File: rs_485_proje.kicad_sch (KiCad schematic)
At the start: 69 parts, among them J1 xt60_female, J10 Extra_pins, J12 P_E_SENSOR_2, J2 RJ45_LED, J3 xt60_female, J4 Led_conn, J5 P_E_SENSOR_1, J6 USB_B_Mini, J7 H_E_sensor_1, J8 H_E_sensor_2, J9 Debug, U1 AP2112K-3.3, U10 FT232RL, U11 USBLC6-2SC6, U2 STM32G030F6Px, U4 ADM2587E, U5 TPS5420D, U7 TLP2161

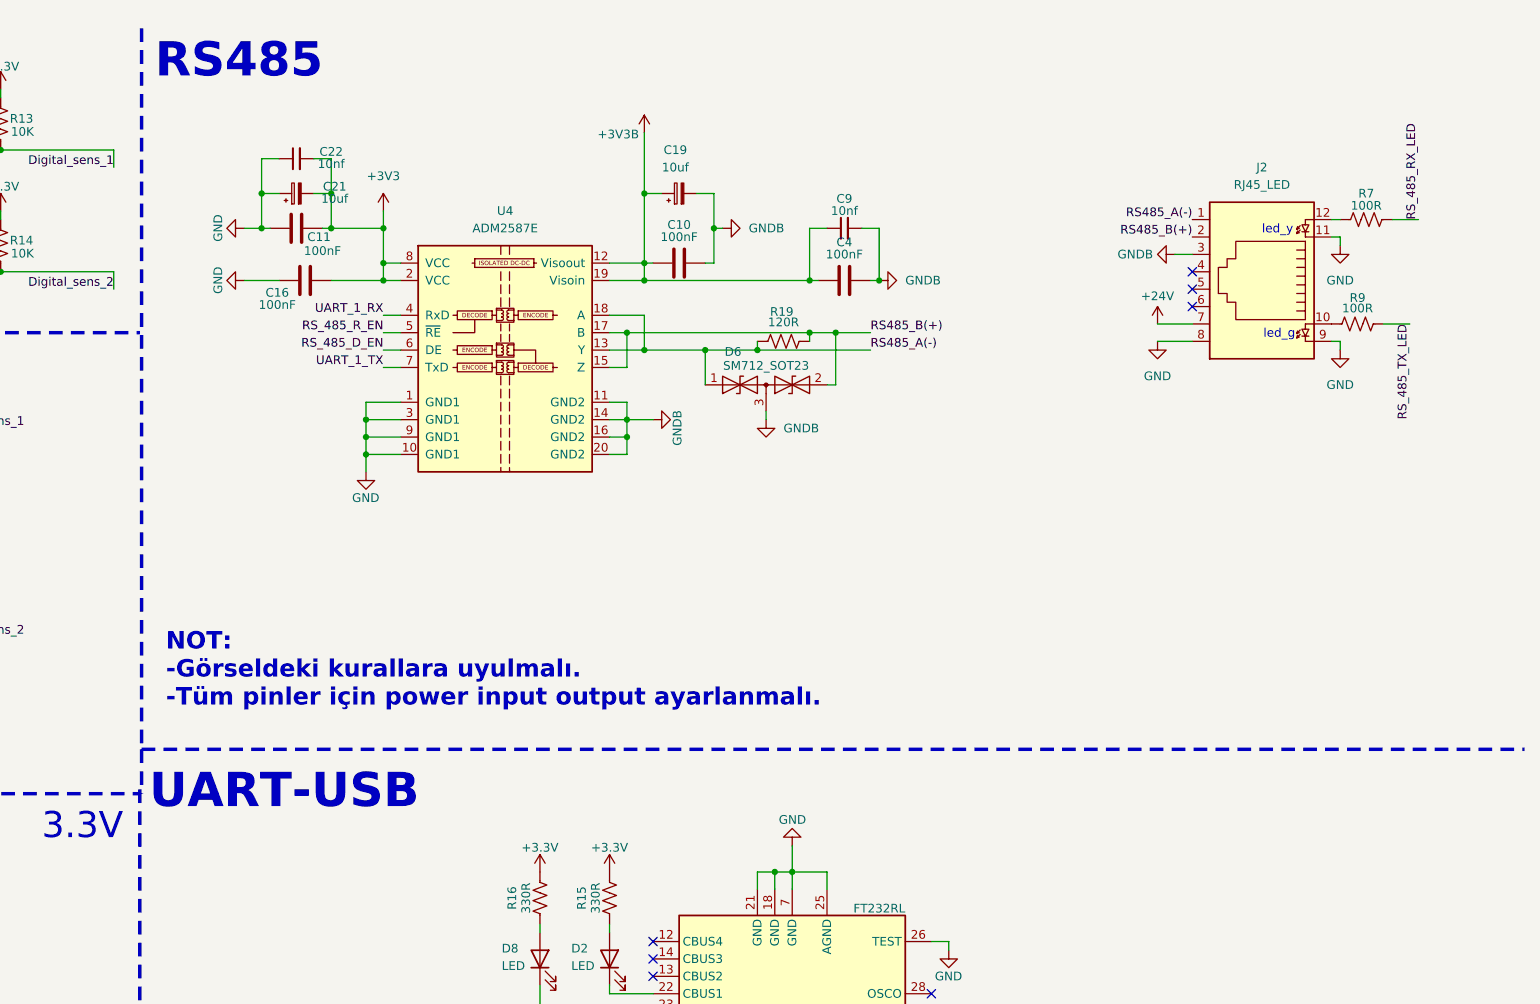
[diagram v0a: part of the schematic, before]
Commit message: 12/05/16:18
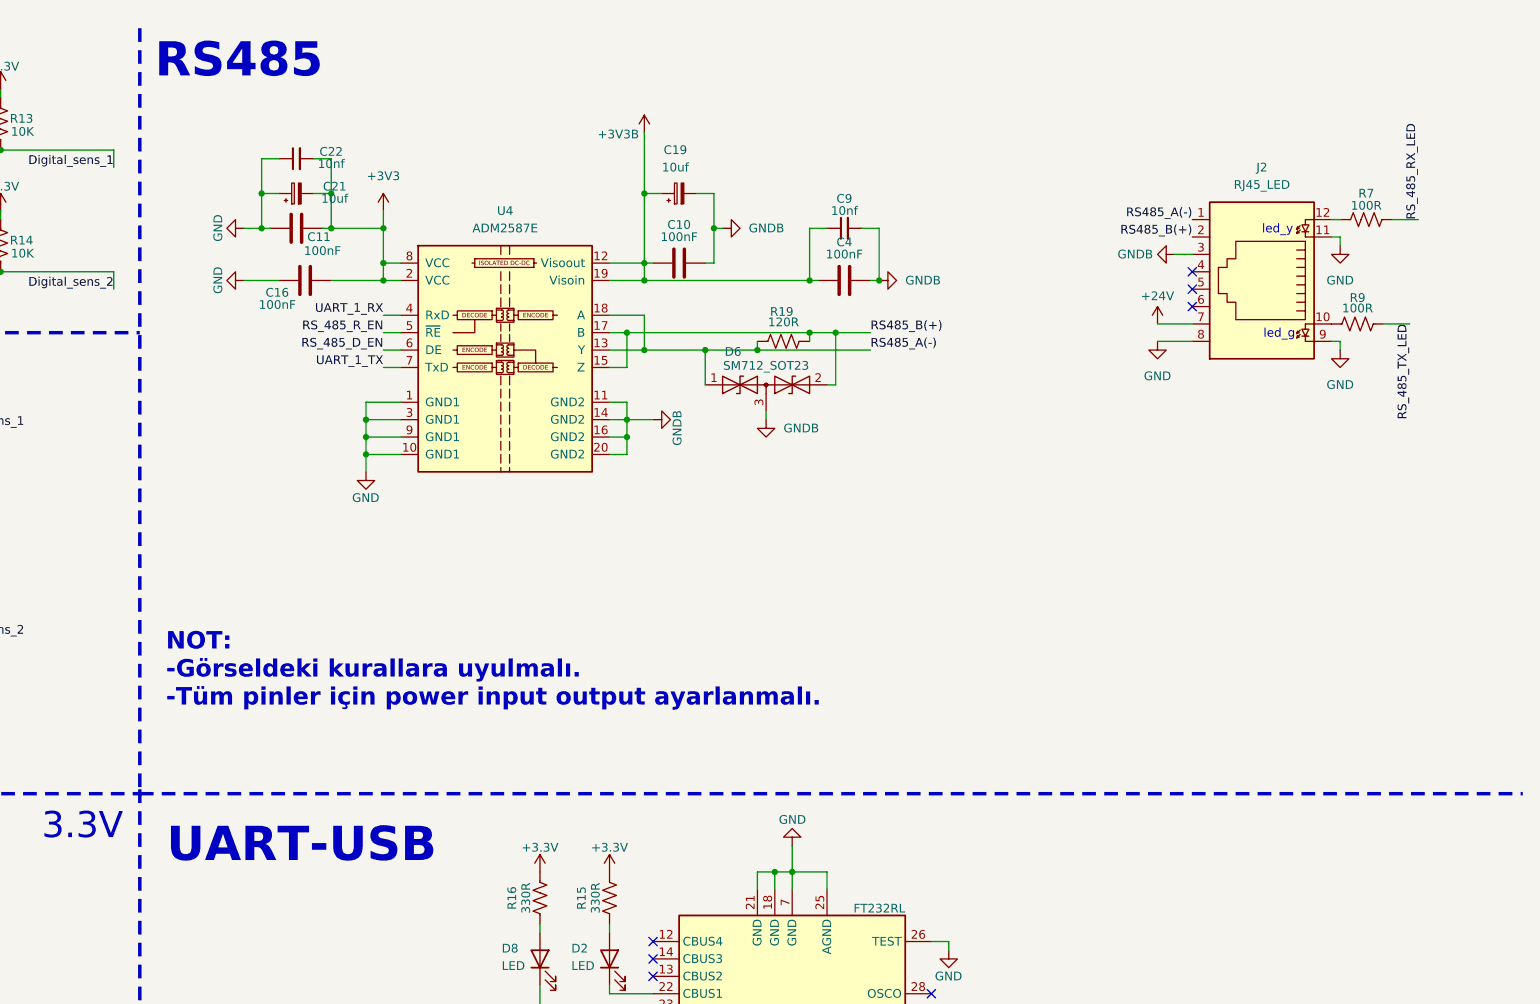
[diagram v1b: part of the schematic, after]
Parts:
- C1, C18, C7, C8: footprint Capacitor_SMD:C_0805_2012Metric -> Capacitor_SMD:C_1206_3216Metric
- C19, C21: footprint Capacitor_SMD:C_0603_1608Metric -> Capacitor_THT:C_Radial_D5.0mm_H11.0mm_P2.00mm
- C2: footprint Capacitor_SMD:C_0805_2012Metric -> Capacitor_THT:C_Radial_D5.0mm_H11.0mm_P2.00mm
- D1: footprint Diode_SMD:D_SMA -> Diode_SMD:D_SMC
- L1: footprint Inductor_THT:L_Radial_D10.0mm_P5.00mm_Fastron_07M -> Inductor_THT:L_Radial_D12.0mm_P5.00mm_Fastron_11P
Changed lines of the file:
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@@
 	(text "UART-USB"
 		(exclude_from_sim no)
-		(at 226.822 124.206 0)
+		(at 229.362 132.08 0)
 		(effects
 			(font
@@
 	(polyline
 		(pts
-			(xy 205.994 117.983) (xy 205.994 124.46)
+			(xy 205.74 124.46) (xy 205.74 124.46)
 		)
 		(stroke
@@
 	(polyline
 		(pts
-			(xy 205.994 12.7) (xy 205.994 117.983)
+			(xy 205.74 12.7) (xy 205.74 124.46)
 		)
 		(stroke
@@
 	(polyline
 		(pts
-			(xy 205.994 117.983) (xy 407.924 117.983)
+			(xy 205.74 124.46) (xy 407.67 124.46)
 		)
 		(stroke
@@
 			)
 		)
-		(property "Footprint" "Capacitor_SMD:C_0805_2012Metric"
+		(property "Footprint" "Capacitor_THT:C_Radial_D5.0mm_H11.0mm_P2.00mm"
 			(at 105.41 154.94 0)
 			(effects
@@
 			)
 		)
-		(property "Footprint" "Capacitor_SMD:C_0805_2012Metric"
+		(property "Footprint" "Capacitor_SMD:C_1206_3216Metric"
 			(at 26.67 154.94 0)
 			(effects
@@
 			)
 		)
-		(property "Footprint" "Inductor_THT:L_Radial_D10.0mm_P5.00mm_Fastron_07M"
+		(property "Footprint" "Inductor_THT:L_Radial_D12.0mm_P5.00mm_Fastron_11P"
 			(at 97.79 147.32 0)
 			(effects
@@
 			)
 		)
-		(property "Footprint" "Capacitor_SMD:C_0603_1608Metric"
+		(property "Footprint" "Capacitor_THT:C_Radial_D5.0mm_H11.0mm_P2.00mm"
 			(at 228.6 36.83 0)
 			(effects
@@
 			)
 		)
-		(property "Footprint" "Capacitor_SMD:C_0603_1608Metric"
+		(property "Footprint" "Capacitor_THT:C_Radial_D5.0mm_H11.0mm_P2.00mm"
 			(at 284.48 36.83 0)
 			(effects
@@
 			)
 		)
-		(property "Footprint" "Capacitor_SMD:C_0805_2012Metric"
+		(property "Footprint" "Capacitor_SMD:C_1206_3216Metric"
 			(at 40.64 154.94 0)
 			(effects
@@
 			)
 		)
-		(property "Footprint" "Diode_SMD:D_SMA"
+		(property "Footprint" "Diode_SMD:D_SMC"
 			(at 84.455 153.67 0)
 			(effects
@@
 			)
 		)
-		(property "Footprint" "Capacitor_SMD:C_0805_2012Metric"
+		(property "Footprint" "Capacitor_SMD:C_1206_3216Metric"
 			(at 151.4348 152.4 0)
 			(effects
@@
 			)
 		)
-		(property "Footprint" "Capacitor_SMD:C_0805_2012Metric"
+		(property "Footprint" "Capacitor_SMD:C_1206_3216Metric"
 			(at 176.8348 152.4 0)
 			(effects
